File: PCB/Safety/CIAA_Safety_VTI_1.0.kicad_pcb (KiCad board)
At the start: 2 copper layers, 95.9 x 90.2 mm, 283 parts, among them J1 HR911105A, J2 SD-CON, P1 JTAG, P2 CAN 2, P3 CAN 1, P4 DC INPUT, P5 USB_OTG, P6 USB_A, P7 CONN_02X32, P8 CAN2, P9 CAN1, Q1 NDS7002A, Q2 NDS7002A, SW1 POWER ON RESET, SW2 WARM RESET, U1 SN65HVD1040, U10 TPS3106K33_DBV_6, U11 LM2596S-5.0, U12 INA210_DCK_6, U13 CH340G, U14 CH376S, U2 PESD1CAN, U3 SN65HVD1040, U4 PESD1CAN, U5 S70FL01GS, U6 Si502, U7 LAN8720A-CP, U8 TMS570LS1227, U9 LM26420, Y1 16MHz, Y2 12MHz, Y3 12MHz

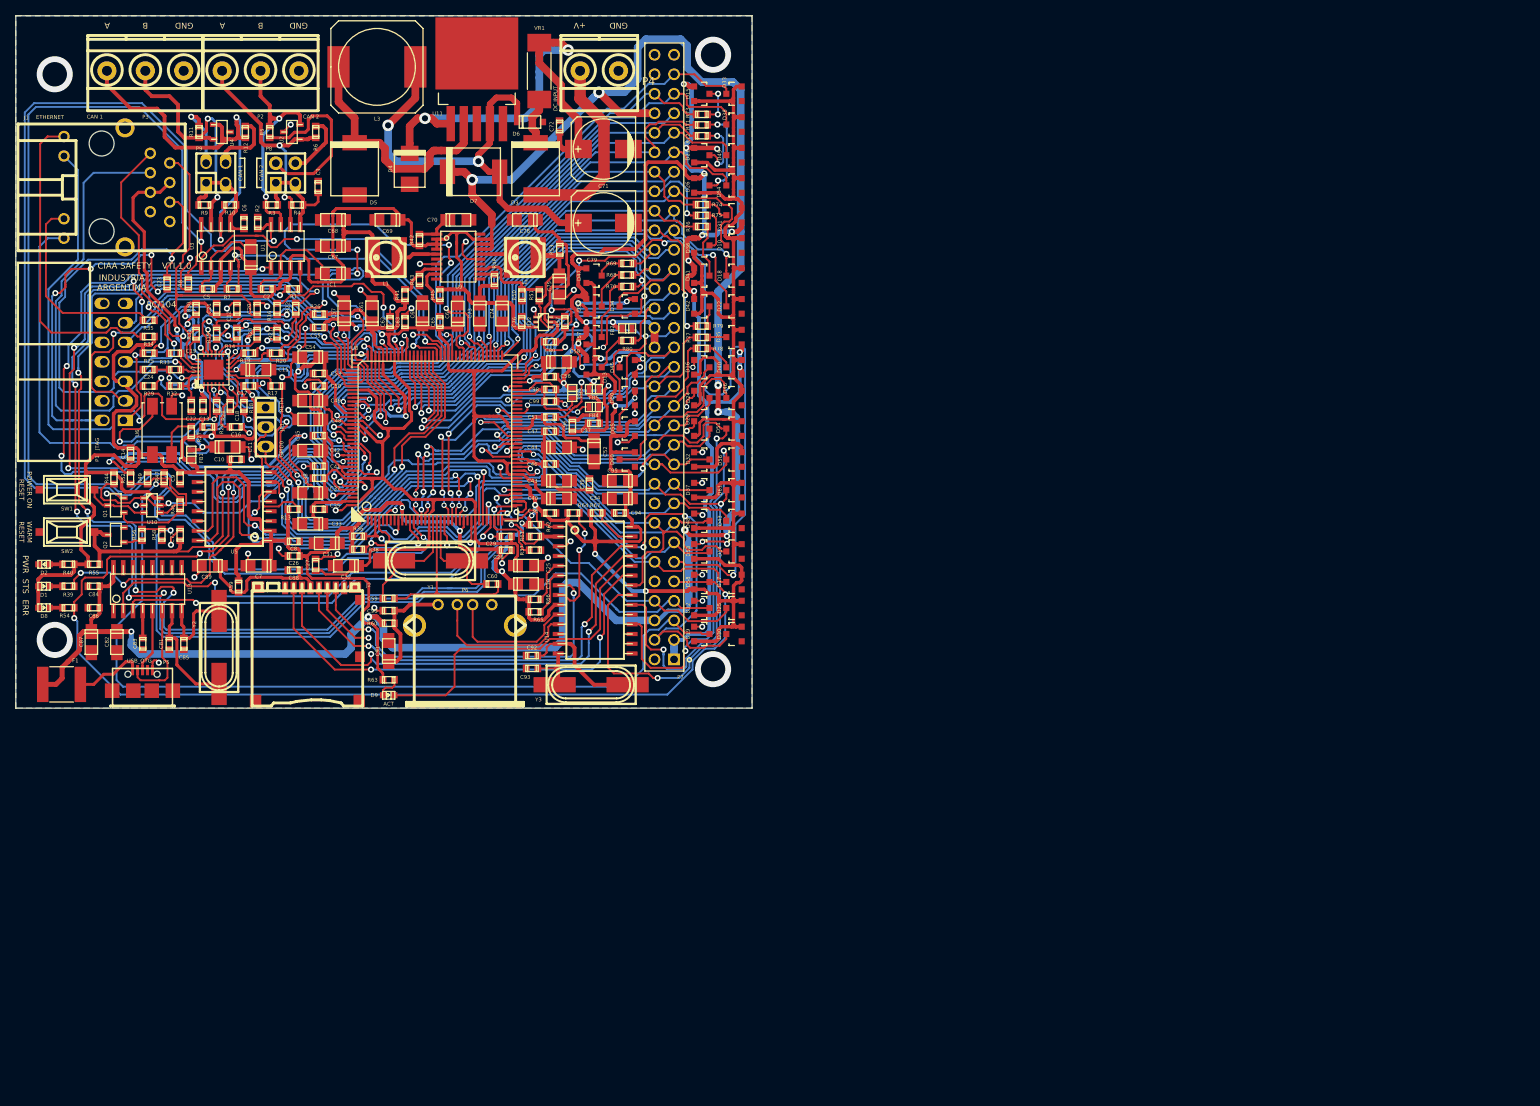
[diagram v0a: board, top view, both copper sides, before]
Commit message: Added Diego Fusari's last version. Changes in texts, title blocks and sheet names.
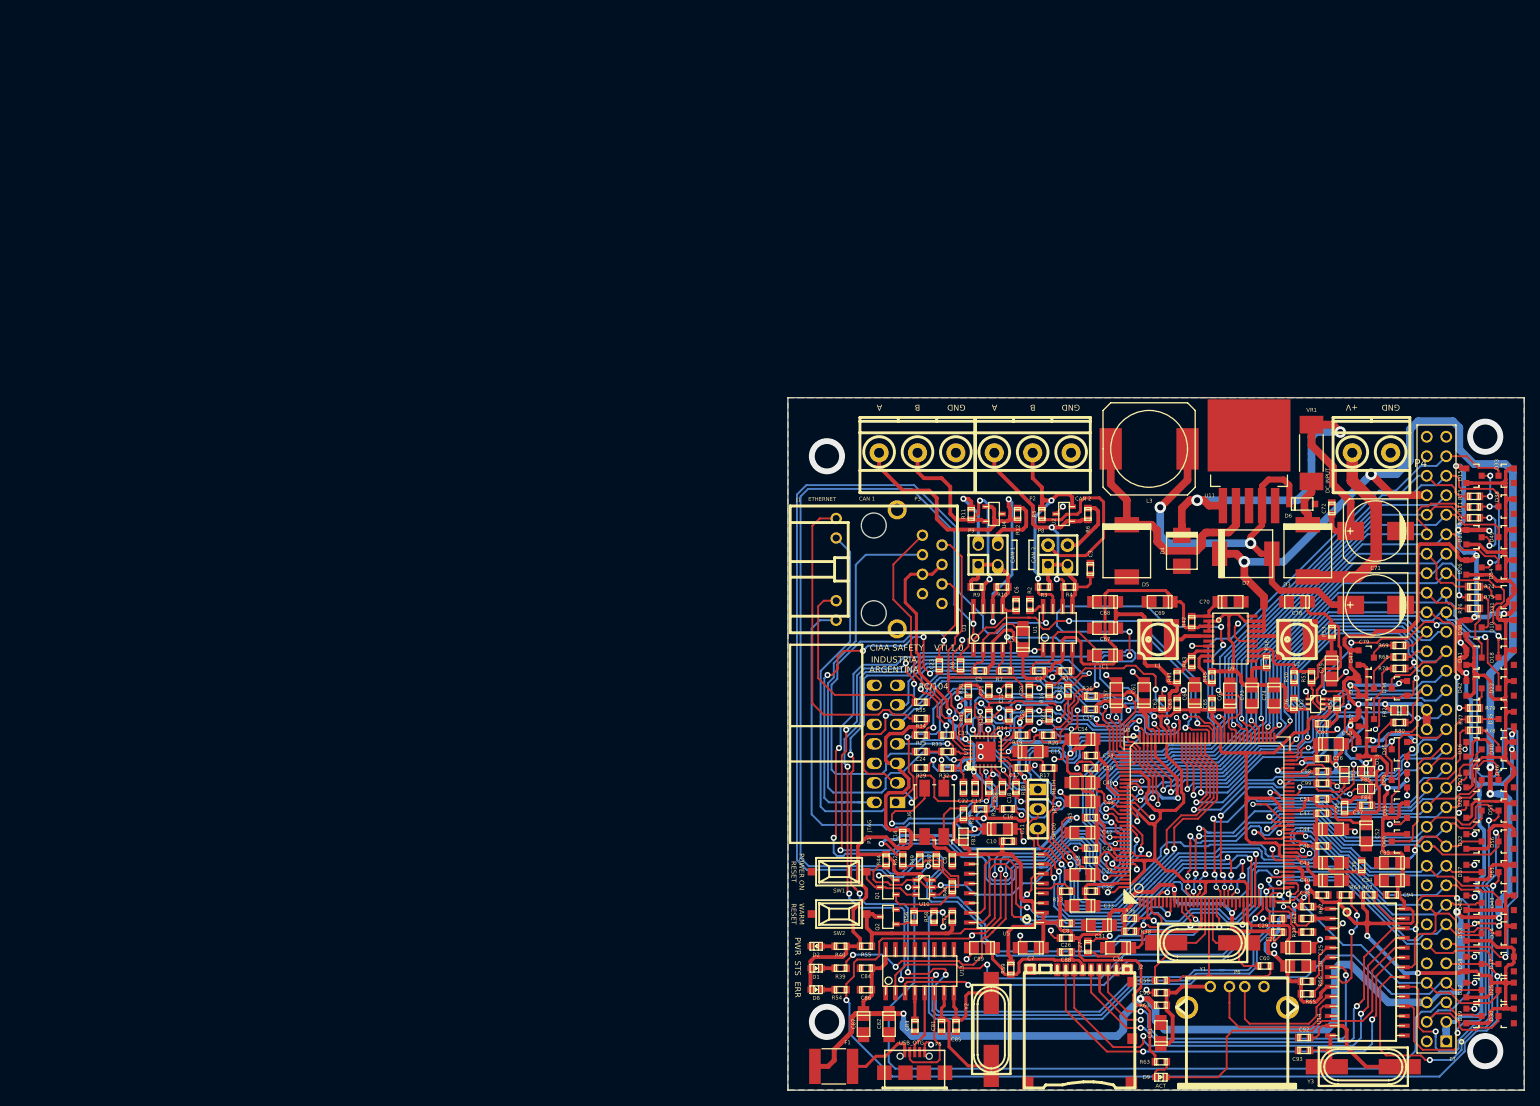
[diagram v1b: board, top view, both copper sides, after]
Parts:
- moved C1 112.2 mm to (141.9, 83.3)
- moved C2 112.2 mm to (133.2, 85.3)
- moved C26 112.2 mm to (136.8, 120.1)
- moved C35 112.2 mm to (140.0, 114.0)
- moved C38 112.2 mm to (140.0, 110.0)
- moved C41 112.2 mm to (140.0, 108.4)
- moved C45 112.2 mm to (140.0, 104.4)
- moved C50 112.2 mm to (140.0, 98.0)
- moved C53 112.2 mm to (140.0, 96.3)
- moved C55 112.2 mm to (140.0, 90.3)
- moved C59 112.2 mm to (149.1, 125.6)
- moved C60 112.2 mm to (162.6, 123.7)
- moved C65 112.2 mm to (155.8, 89.6)
- moved C67 112.2 mm to (141.9, 79.7)
- moved C68 112.2 mm to (141.9, 76.3)
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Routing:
- net (no net): vias 5 -> 7
